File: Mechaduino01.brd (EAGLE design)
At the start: 41.9 x 41.9 mm, 64 parts, among them IC1 SAMD21G18A-AUT, Q1 BSS138, Q2 NFET, Q3 BSS138, Q4 BSS138, Q5 BSS138, U1 TLV70233PDBVR, Y1 32,768Khz

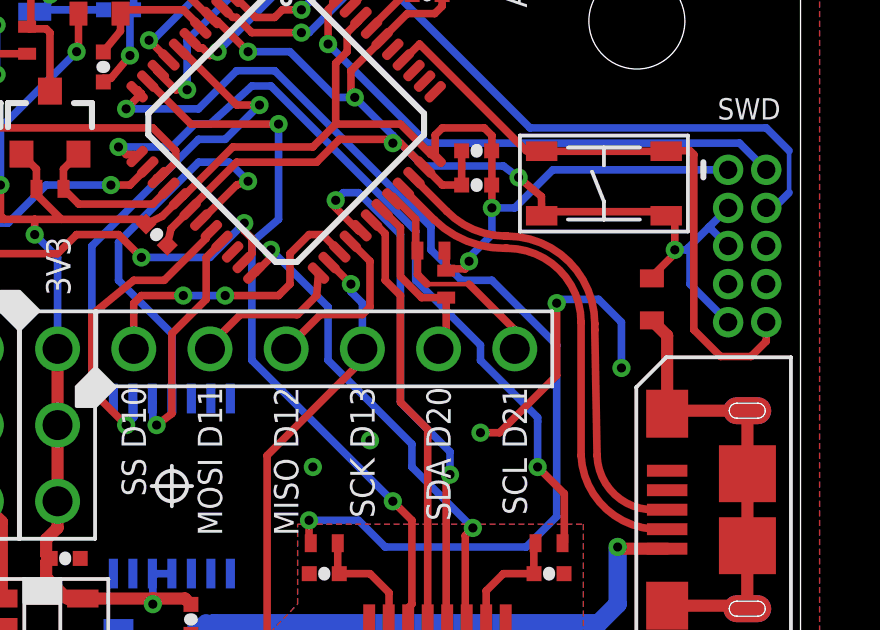
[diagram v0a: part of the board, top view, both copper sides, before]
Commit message: updated caps
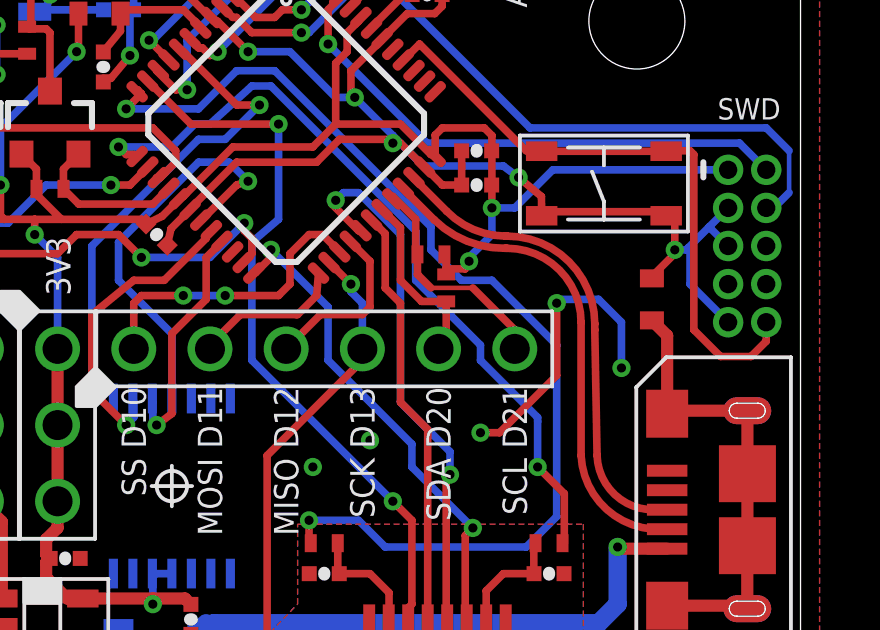
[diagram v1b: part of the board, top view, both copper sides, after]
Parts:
- C7, C8: value 22pF -> 18pF
- moved R7 0.13 mm to (29.6, 28.7)
- moved R8 0.13 mm to (30.1, 27.6)
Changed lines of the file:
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@@
 <element name="C2" library="swift" package="0402-CAP" value="0.1uF" x="31.115" y="30.988" smashed="yes" rot="R180"/>
 <element name="C5" library="swift" package="0402-CAP" value="0.1uF" x="18.669" y="34.925" smashed="yes" rot="R270"/>
-<element name="C7" library="swift" package="0402-CAP" value="22pF" x="19.177" y="38.1" smashed="yes" rot="MR0"/>
-<element name="C8" library="swift" package="0402-CAP" value="22pF" x="19.177" y="36.83" smashed="yes" rot="MR0"/>
+<element name="C7" library="swift" package="0402-CAP" value="18pF" x="19.177" y="38.1" smashed="yes" rot="MR0"/>
+<element name="C8" library="swift" package="0402-CAP" value="18pF" x="19.177" y="36.83" smashed="yes" rot="MR0"/>
 <element name="LED1" library="Opto" package="CHIPLED_0805" value="Green" x="3.937" y="23.749" smashed="yes" rot="R270">
 <attribute name="CASE" value="" x="3.937" y="23.749" size="1.778" layer="27" rot="R270" display="off"/>
@@
 <attribute name="PART_NUMBER" value="KPT-2012YC" x="3.937" y="23.749" size="1.778" layer="27" rot="R270" display="off"/>
 </element>
-<element name="R7" library="adafruit" package="R0402-VISHAY" value="4.7K" x="29.591" y="28.8036" smashed="yes"/>
-<element name="R8" library="adafruit" package="R0402-VISHAY" value="4.7K" x="30.099" y="27.686" smashed="yes" rot="R90"/>
+<element name="R7" library="adafruit" package="R0402-VISHAY" value="4.7K" x="29.591" y="28.6766" smashed="yes"/>
+<element name="R8" library="adafruit" package="R0402-VISHAY" value="4.7K" x="30.099" y="27.559" smashed="yes" rot="R90"/>
 <element name="C1" library="swift" package="0402-CAP" value="0.1uF" x="31.115" y="32.131" smashed="yes" rot="R180"/>
 <element name="C3" library="swift" package="0402-CAP" value="0.1uF" x="20.447" y="29.337" smashed="yes" rot="R135"/>
@@
 <contactref element="R1" pad="2"/>
 <wire x1="30.099" y1="28.194" x2="30.099" y2="28.7456" width="0.254" layer="1"/>
-<wire x1="30.099" y1="28.7456" x2="30.041" y2="28.8036" width="0.254" layer="1"/>
-<wire x1="30.861" y1="28.448" x2="30.734" y2="28.575" width="0.254" layer="16"/>
-<wire x1="30.861" y1="28.321" x2="30.861" y2="28.448" width="0.254" layer="1"/>
-<wire x1="30.734" y1="28.194" x2="30.861" y2="28.321" width="0.254" layer="1"/>
+<wire x1="30.099" y1="28.7456" x2="30.041" y2="28.6766" width="0.254" layer="1"/>
+<wire x1="30.734" y1="28.194" x2="30.861" y2="28.448" width="0.254" layer="1"/>
 <wire x1="30.099" y1="28.194" x2="30.734" y2="28.194" width="0.254" layer="1"/>
-<wire x1="30.099" y1="28.194" x2="30.099" y2="28.136" width="0.254" layer="1"/>
+<wire x1="30.099" y1="28.194" x2="30.099" y2="28.009" width="0.254" layer="1"/>
 <via x="30.861" y="28.448" extent="1-16" drill="0.3048" diameter="0.254"/>
 <wire x1="31.623" y1="29.337" x2="31.623" y2="30.226" width="0.254" layer="16"/>
@@
 <wire x1="29.464" y1="16.2291" x2="29.4827" y2="16.2104" width="0.254" layer="1"/>
 <wire x1="27.611103125" y1="29.820340625" x2="28.067" y2="29.36444375" width="0.254" layer="1"/>
-<wire x1="28.067" y1="29.36444375" x2="28.067" y2="27.813" width="0.254" layer="1"/>
-<wire x1="28.067" y1="27.813" x2="28.575" y2="27.305" width="0.254" layer="1"/>
-<wire x1="28.575" y1="27.305" x2="28.575" y2="23.749" width="0.254" layer="1"/>
+<wire x1="28.067" y1="29.36444375" x2="28.067" y2="27.559" width="0.254" layer="1"/>
+<wire x1="28.067" y1="27.559" x2="28.575" y2="27.051" width="0.254" layer="1"/>
+<wire x1="28.575" y1="27.051" x2="28.575" y2="23.749" width="0.254" layer="1"/>
 <wire x1="28.575" y1="23.749" x2="29.4827" y2="22.8413" width="0.254" layer="1"/>
 <wire x1="29.4827" y1="22.8413" x2="29.4827" y2="16.2104" width="0.254" layer="1"/>
@@
 <contactref element="R8" pad="1"/>
 <contactref element="J3" pad="P$5"/>
-<wire x1="30.099" y1="27.236" x2="29.279" y2="27.236" width="0.254" layer="1"/>
-<wire x1="29.279" y1="27.236" x2="28.575" y2="27.94" width="0.254" layer="1"/>
-<wire x1="28.575" y1="27.94" x2="28.575" y2="29.56355" width="0.254" layer="1"/>
+<wire x1="30.099" y1="27.109" x2="29.279" y2="27.109" width="0.254" layer="1"/>
+<wire x1="29.279" y1="27.109" x2="28.575" y2="27.813" width="0.254" layer="1"/>
+<wire x1="28.575" y1="27.813" x2="28.575" y2="29.56355" width="0.254" layer="1"/>
 <wire x1="28.575" y1="29.56355" x2="27.96465625" y2="30.17389375" width="0.254" layer="1"/>
 <wire x1="29.845" y1="25.527" x2="30.099" y2="25.781" width="0.254" layer="1"/>
-<wire x1="30.099" y1="25.781" x2="30.099" y2="27.236" width="0.254" layer="1"/>
+<wire x1="30.099" y1="25.781" x2="30.099" y2="27.109" width="0.254" layer="1"/>
 </signal>
 <signal name="ARDUINO_D21_SCL">
@@
 <contactref element="R7" pad="1"/>
 <contactref element="J3" pad="P$6"/>
-<wire x1="29.083" y1="28.829" x2="29.141" y2="28.8036" width="0.254" layer="1"/>
+<wire x1="29.083" y1="28.829" x2="29.141" y2="28.6766" width="0.254" layer="1"/>
 <wire x1="29.083" y1="29.845" x2="29.083" y2="28.829" width="0.254" layer="1"/>
 <wire x1="28.321" y1="30.607" x2="29.083" y2="29.845" width="0.254" layer="1"/>
 <wire x1="28.321" y1="30.607" x2="28.318209375" y2="30.527446875" width="0.254" layer="1"/>
-<wire x1="29.141" y1="28.8036" x2="29.141" y2="28.009" width="0.254" layer="1"/>
-<wire x1="29.141" y1="28.009" x2="29.464" y2="27.686" width="0.254" layer="1"/>
+<wire x1="29.141" y1="28.6766" x2="29.141" y2="28.009" width="0.254" layer="1"/>
+<wire x1="29.141" y1="28.009" x2="29.591" y2="27.559" width="0.254" layer="1"/>
 <wire x1="32.385" y1="25.527" x2="32.385" y2="26.162" width="0.254" layer="1"/>
-<wire x1="32.385" y1="26.162" x2="30.861" y2="27.686" width="0.254" layer="1"/>
-<wire x1="29.464" y1="27.686" x2="30.861" y2="27.686" width="0.1524" layer="1"/>
+<wire x1="32.385" y1="26.162" x2="30.988" y2="27.559" width="0.254" layer="1"/>
+<wire x1="29.591" y1="27.559" x2="30.988" y2="27.559" width="0.1524" layer="1"/>
 </signal>
 <signal name="HEADER_MOSI">
